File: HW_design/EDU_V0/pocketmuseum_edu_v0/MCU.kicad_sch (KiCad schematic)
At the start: 34 parts, among them J201 TF-015, J205 BM04B-SRSS-TB, J206 BM04B-SRSS-TB, SW201 PTS810SJG250, U201 ESP32-C6-MINI-1/U

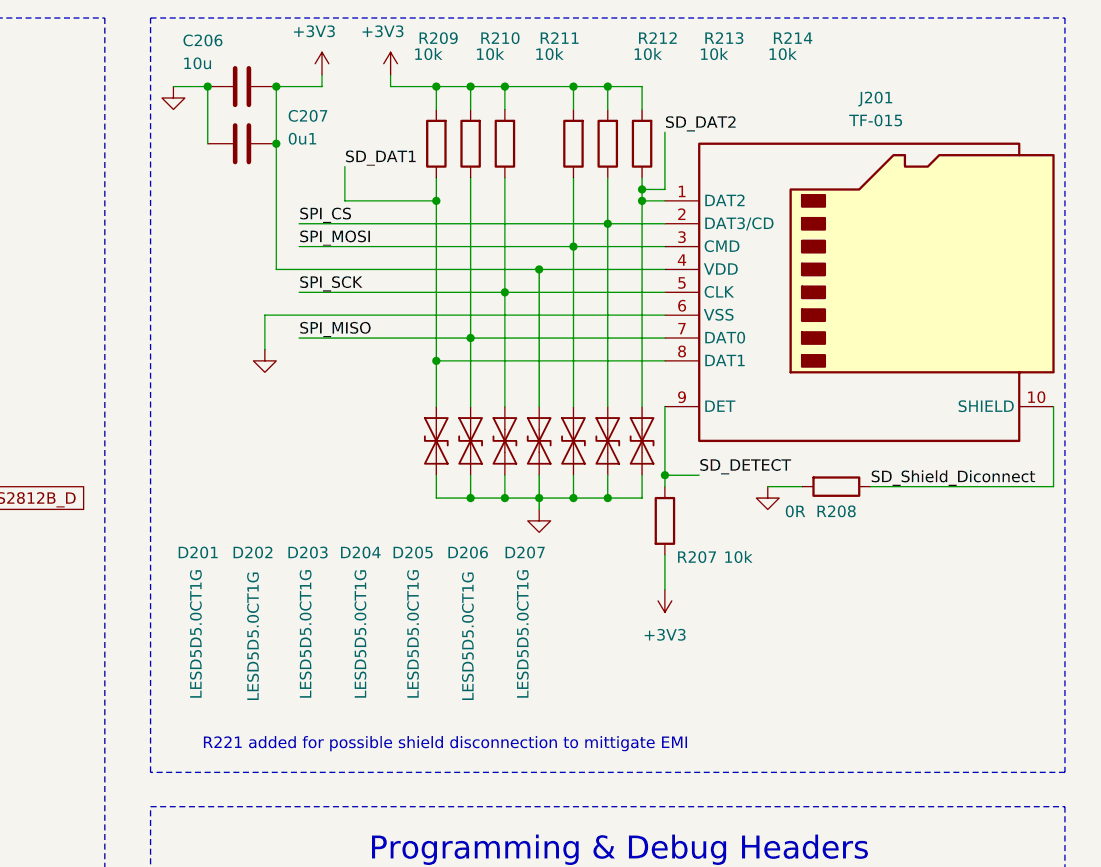
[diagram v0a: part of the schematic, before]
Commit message: Diagram review complete
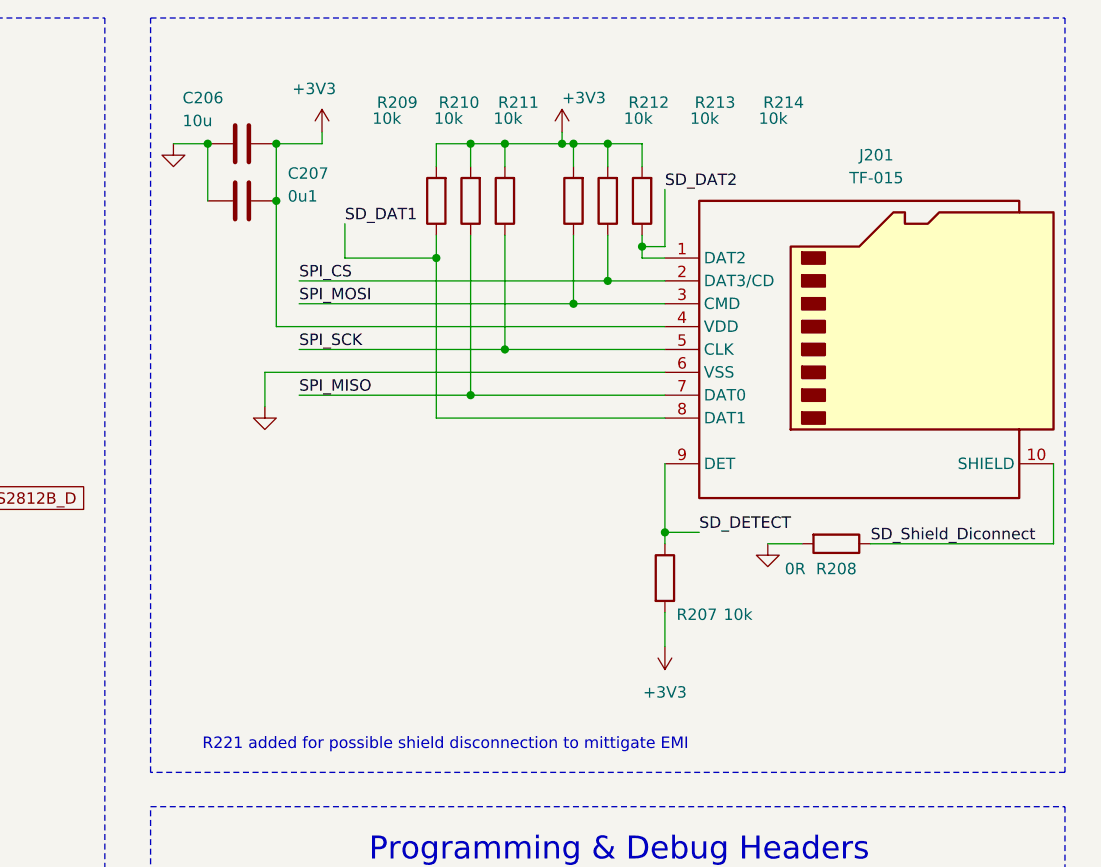
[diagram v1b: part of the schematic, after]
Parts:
- removed D201, D202, D203, D204, D205, D206, D207: LESD5D5.0CT1G, Diode_SMD:D_SOD-523, symbol Diode:ESD9B5.0ST5G
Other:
- moved on the sheet: C206, C207, J201, R207, R208, R209, R210, R211, R212, R213, R214
